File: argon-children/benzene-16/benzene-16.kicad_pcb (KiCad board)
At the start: 2 copper layers, 25 x 30 mm, 19 parts, among them J1 Conn2, J2 Conn1, U1 DIP-8, U2 LMC555, U3 DIP-16

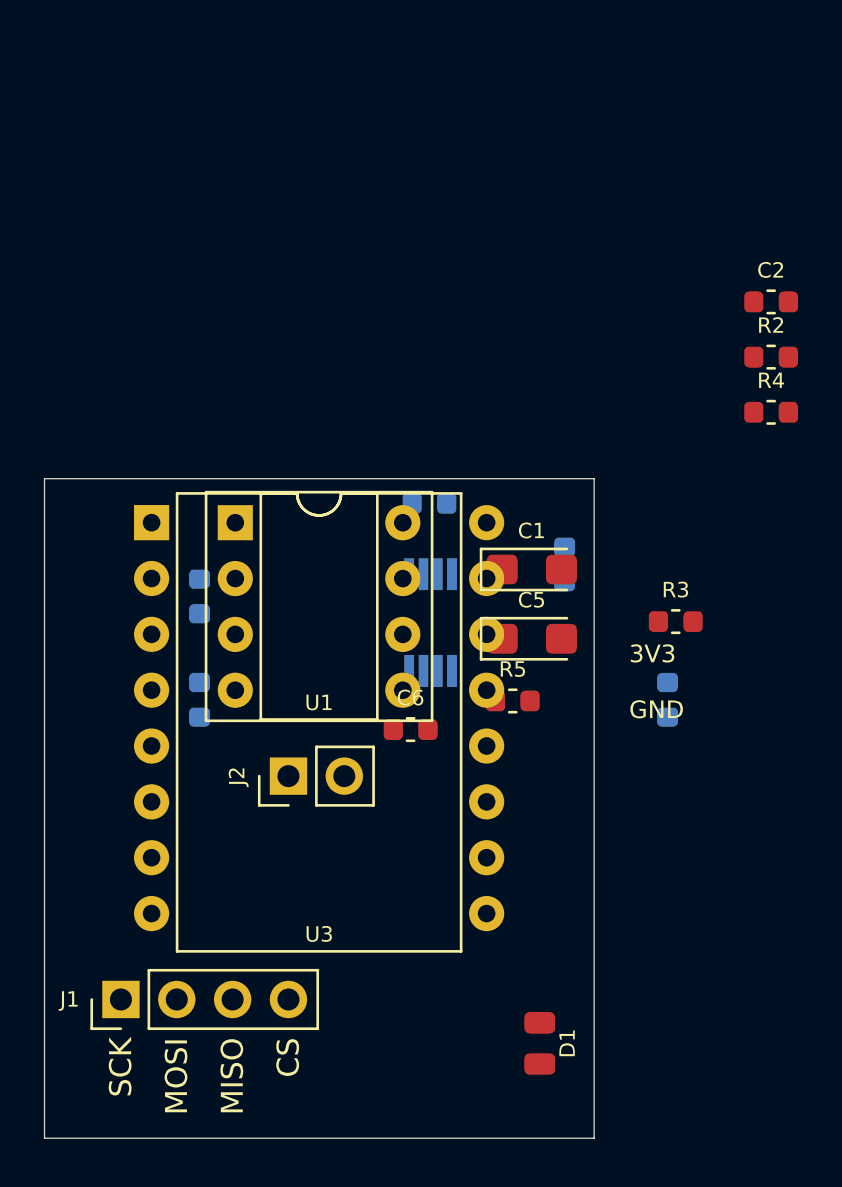
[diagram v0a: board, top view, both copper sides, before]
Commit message: Benzene PCB
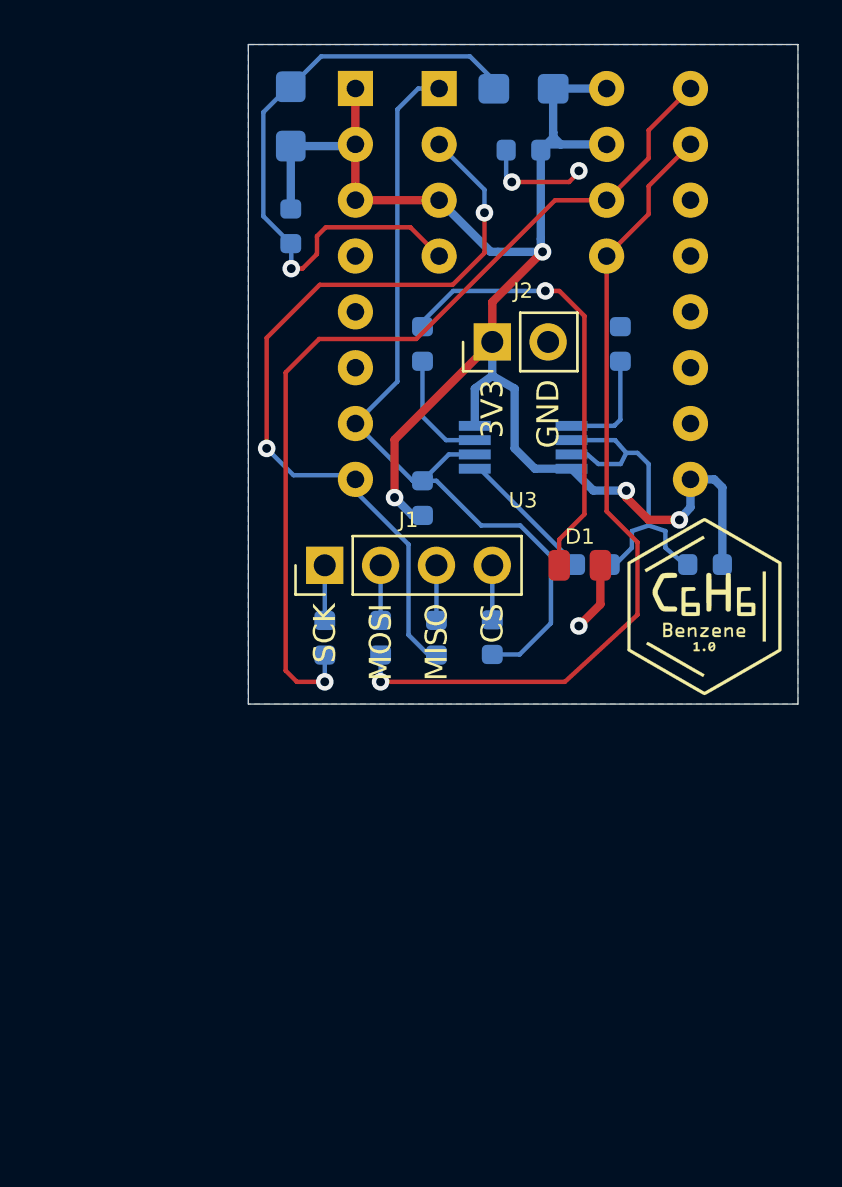
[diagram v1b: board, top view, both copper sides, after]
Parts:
- added G***: LOGO, benzene:benzene-duze, F.Cu at (116.0, 75.8)
- C1, C5: footprint Capacitor_Tantalum_SMD:CP_EIA-3216-18_Kemet-A -> argon:CP_EIA-3216-18_Kemet-A; moved to B.Cu
- C2, C6, R2, R3, R4, R5: moved to B.Cu
- U1: footprint benzene:DIP-8_W7.62mm_Socket -> benzene:DIP-8_W7.62mm_Socket_wihtout_lines
- U3: footprint benzene:DIP-16_W15.24mm -> benzene:DIP-16_W15.24mm_without_lines
- moved C5 26.2 mm to (97.2, 53.5), turned to 90 degrees
- moved R6 23.8 mm to (116.0, 73.9), turned to 180 degrees
- moved C6 23.5 mm to (97.2, 58.5), turned to 90 degrees
- moved C1 21.9 mm to (107.8, 52.3), turned to 180 degrees
- moved D1 21.8 mm to (110.3, 73.9), turned to 180 degrees
- moved U1 21.8 mm to (103.9, 52.3)
- moved U3 21.8 mm to (100.1, 52.3)
- moved J1 21.8 mm to (98.7, 73.9)
- moved J2 21.8 mm to (106.4, 63.8)
- moved R4 20.5 mm to (101.3, 77.2), turned to 90 degrees
- moved R2 18.0 mm to (106.4, 77.2), turned to 90 degrees
- moved C2 13.2 mm to (107.8, 55.1)
- moved R1 11.1 mm to (103.2, 70.9), turned to 90 degrees
- moved R3 10.9 mm to (103.8, 77.2), turned to 90 degrees
- moved C3 10.3 mm to (112.2, 63.9), turned to 270 degrees
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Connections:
- U2 pad 2: (no net) -> CS
- U3 pad 1: (no net) -> V3V3
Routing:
- net V3V3: track 0.00 -> 74.6 mm, vias 0 -> 4
- net GND: track 0.00 -> 43.2 mm, vias 0 -> 4
- net SCK: track 0.00 -> 41.3 mm, vias 0 -> 1
- net CS: track 0.00 -> 37.9 mm
- net MOSI: track 0.00 -> 37.7 mm, vias 0 -> 1
- net MISO: track 0.00 -> 36.7 mm, vias 0 -> 2
- net Net-(D1-Pad2): track 0.00 -> 20.5 mm, vias 0 -> 1
- net Net-(C4-Pad1): track 0.00 -> 15.1 mm
- net Net-(R7-Pad1): track 0.00 -> 5.34 mm
- net Net-(C3-Pad2): track 0.00 -> 4.99 mm
- net Net-(J1-Pad3): track 0.00 -> 2.51 mm
- net Net-(J1-Pad2): track 0.00 -> 2.51 mm
- net Net-(J1-Pad1): track 0.00 -> 2.51 mm
- net Net-(J1-Pad4): track 0.00 -> 2.48 mm
- added copper zone on B.Cu, net GND
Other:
- net class Default: clearance 0.127 -> 0.1524
- net class zasilanie: clearance 0.381 -> 0.1524
- rule trace_clearance: 0.127 -> 0.1524
